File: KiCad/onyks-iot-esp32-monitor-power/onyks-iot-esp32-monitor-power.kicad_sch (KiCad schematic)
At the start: 51 parts, among them J1 Uart_con, J10 PAD, J11 PAD, J12 PAD, J13 PAD, J14 +3V3_PAD, J15 +5V_PAD, J16 FOUT_conn, J17 Ground, J2 Jtag_con, J3 UART_ONYKS, J4 I_SENS_IN, J5 I_SENS_OUT, J6 MAIN_VOLTAGE_INPUT, J7 Conn_01x02, J8 Screw_Terminal_01x03, J9 UART2, K1 SANYOU_SRD_Form_C, Q1 SS8050, Q2 SS8050, Q3 MMBT2222A, SW1 reset, T1 2mA-2mA transformer, U1 ESP32-WROOM-32D, U2 ADS1115IDGS, U3 ACS712xLCTR-30A, U4 TLV75733PDBV

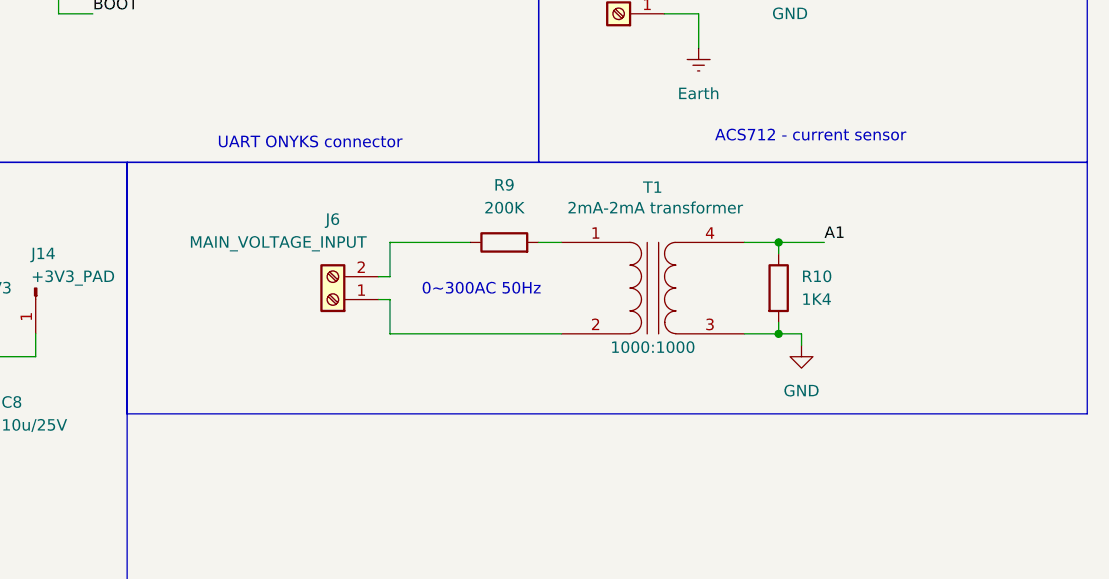
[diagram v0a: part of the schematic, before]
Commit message: fab files v1
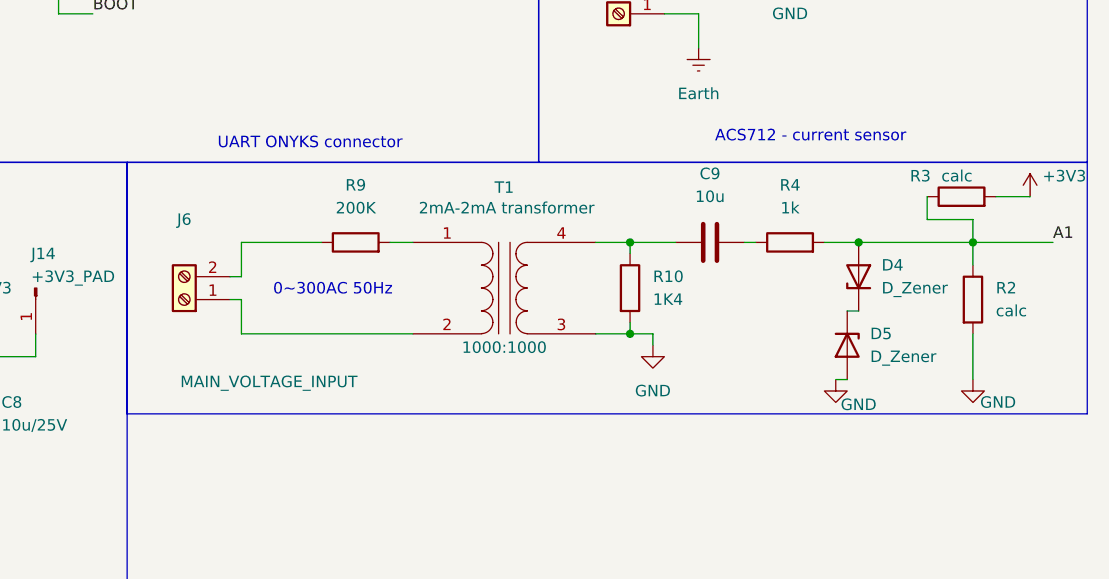
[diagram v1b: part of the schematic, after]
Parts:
- added C9: 10u, Capacitor_SMD:C_0805_2012Metric, symbol Device:C
- added D4, D5: D_Zener, Diode_SMD:D_0805_2012Metric, symbol Device:D_Zener
- added R2, R3: calc, Resistor_SMD:R_0805_2012Metric, symbol Device:R
- added R4: 1k, Resistor_SMD:R_0805_2012Metric, symbol Device:R
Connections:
- net +3V3: now also R3.2
- net A1: now also D4.2 (A), R2.1, R3.1, R4.2; no longer R10.1, T1.4 (SB)
- net GND: now also D5.2 (A), R2.2
- new net: C9.1, R10.1, T1.4 (SB)
- new net: C9.2, R4.1
- new net: D4.1 (K), D5.1 (K)
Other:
- moved on the sheet: J6, R10, R9, T1
